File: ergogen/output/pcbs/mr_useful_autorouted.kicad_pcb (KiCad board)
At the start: 2 copper layers, 57 x 95 mm, 37 parts

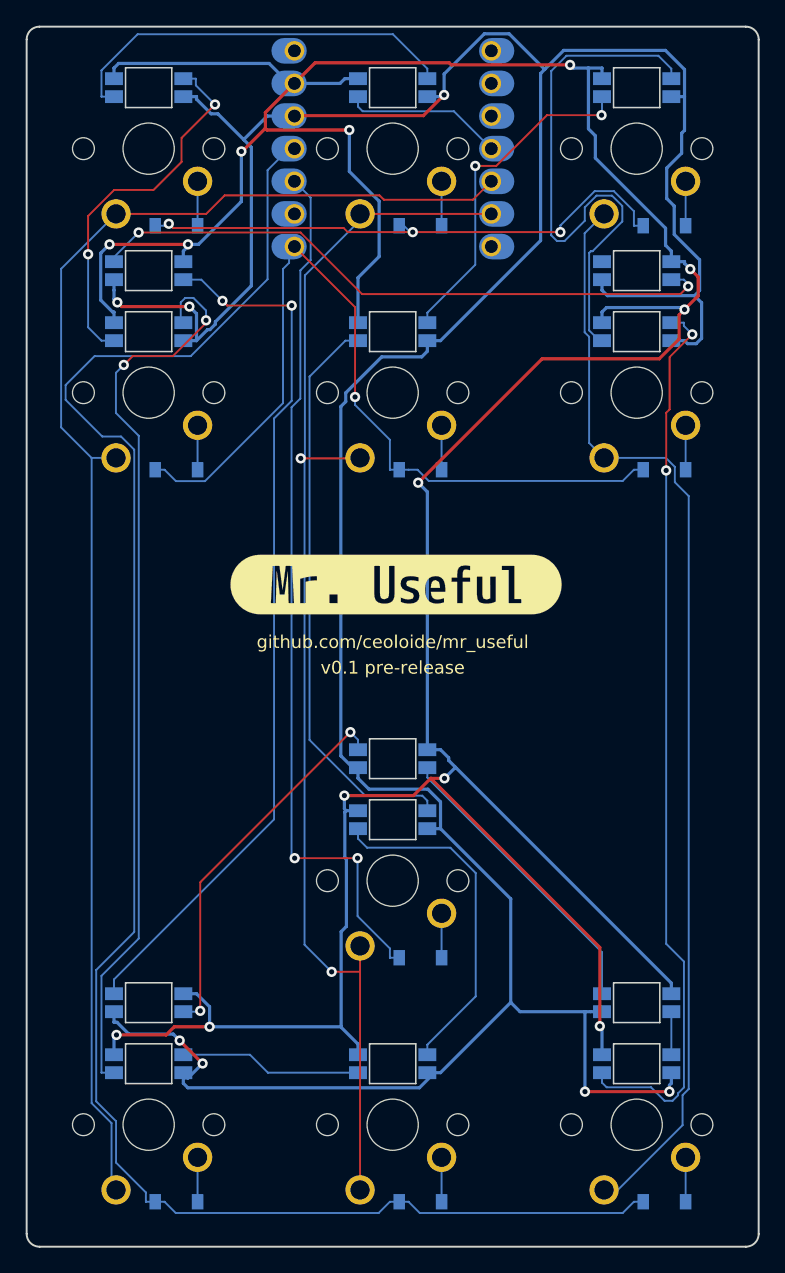
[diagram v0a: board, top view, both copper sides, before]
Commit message: Update assets
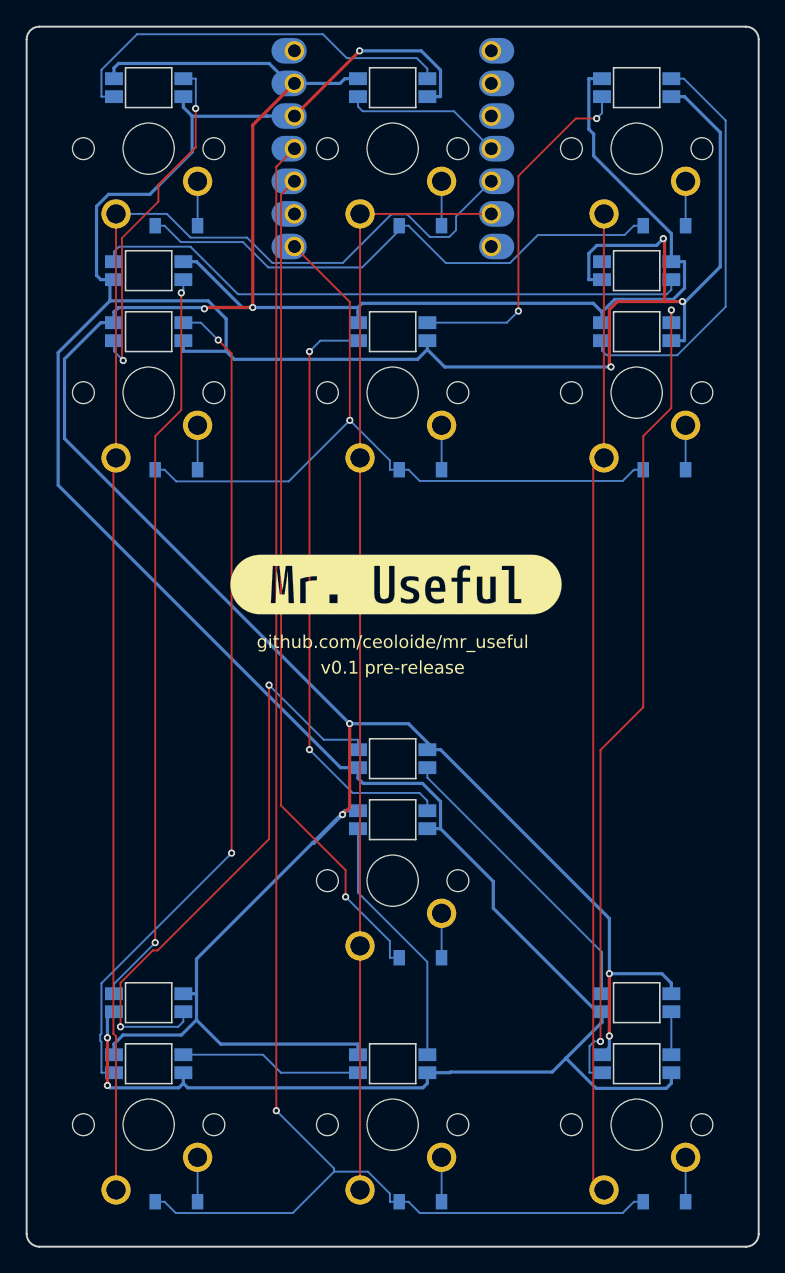
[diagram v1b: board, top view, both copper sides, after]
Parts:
- D1, D10, D2, D3, D4, D5, D6, D7, D8, D9: footprint ComboDiode -> ceoloide:diode_tht_sod123
- LED1, LED10, LED2, LED3, LED4, LED5, LED6, LED7, LED8, LED9: footprint ceoloide:YS-SK6812MINI-E (per-key) -> ceoloide:led_SK6812mini-e (per-keysingle-side)
- LED11, LED12, LED13, LED14, LED15: footprint ceoloide:YS-SK6812MINI-E (underglow) -> ceoloide:led_SK6812mini-e (underglowsingle-side)
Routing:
- net GND: track 289.4 -> 258.5 mm, vias 13 -> 6
- net ULED_2: track 29.5 -> 46.9 mm
- net VCC: track 266.6 -> 282.6 mm, vias 7 -> 6
- net R0: track 140.1 -> 124.3 mm, vias 0 -> 1
- net LED_8: track 44.1 -> 32.2 mm
- net C1: track 98.5 -> 86.6 mm, vias 2 -> 0
- net ULED_3: track 68.6 -> 57.8 mm
- net C2: track 86.2 -> 76.7 mm
- net R3: track 66.5 -> 58.8 mm
- net LED_5: track 26.8 -> 19.8 mm
- net LED_9: track 70.5 -> 64.3 mm
- net LED_3: track 71.2 -> 66.0 mm
- net R1: track 68.8 -> 65.5 mm, vias 2 -> 1
- net ULED_4: track 49.7 -> 46.8 mm, vias 2 -> 0
- net LED_2: track 29.3 -> 27.2 mm
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
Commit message: Update assets
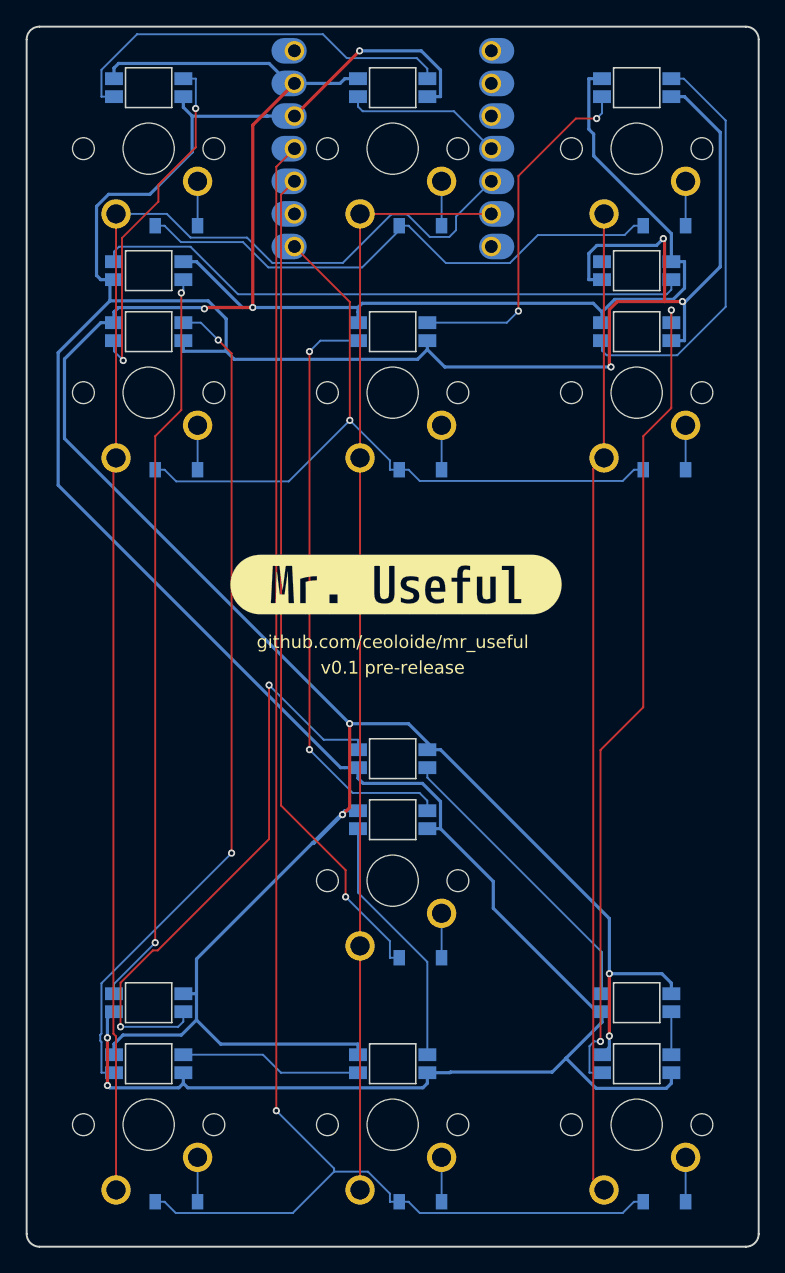
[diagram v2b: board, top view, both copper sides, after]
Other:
- net class Default removed
